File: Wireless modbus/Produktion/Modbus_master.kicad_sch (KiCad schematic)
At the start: 76 parts, among them IC1 LoRa-E5, J1 Screw_Terminal_01x03, J2 XKNANO-113, J3 Conn_01x04_Pin, J4 Conn_Coaxial, J5 Screw_Terminal_01x04, J6 AVR-ISP-6, Q1 BC847CW, Q2 BC847CW, SW1 TL3305AF260QG, U1 ATmega2560-16A, U2 SP485EN-L/TR, U3 L7805, U4 SIM7080G, U5 LSF0204PW-Q100J, Y1 ABM3B-8.000MHZ-10-1-U-T

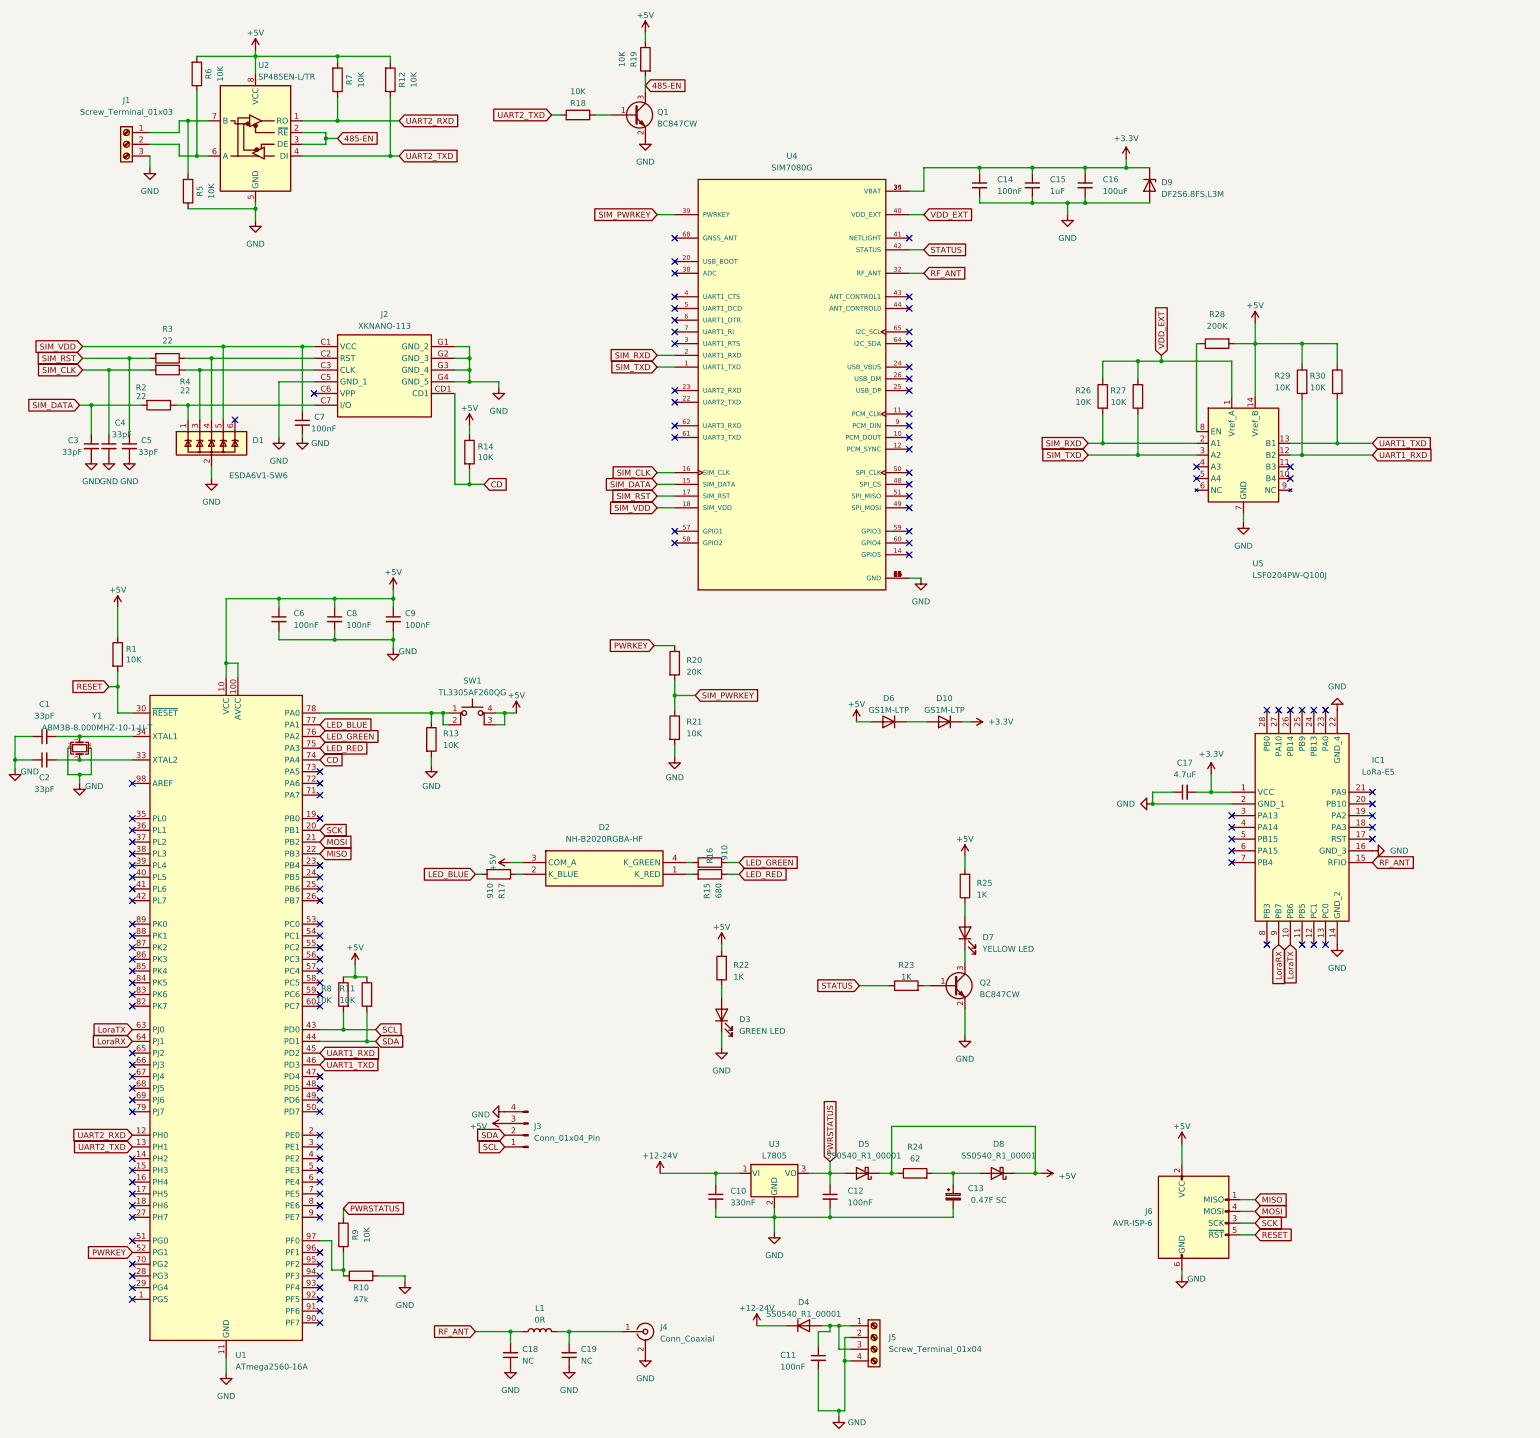
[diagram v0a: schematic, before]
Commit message: Ændring
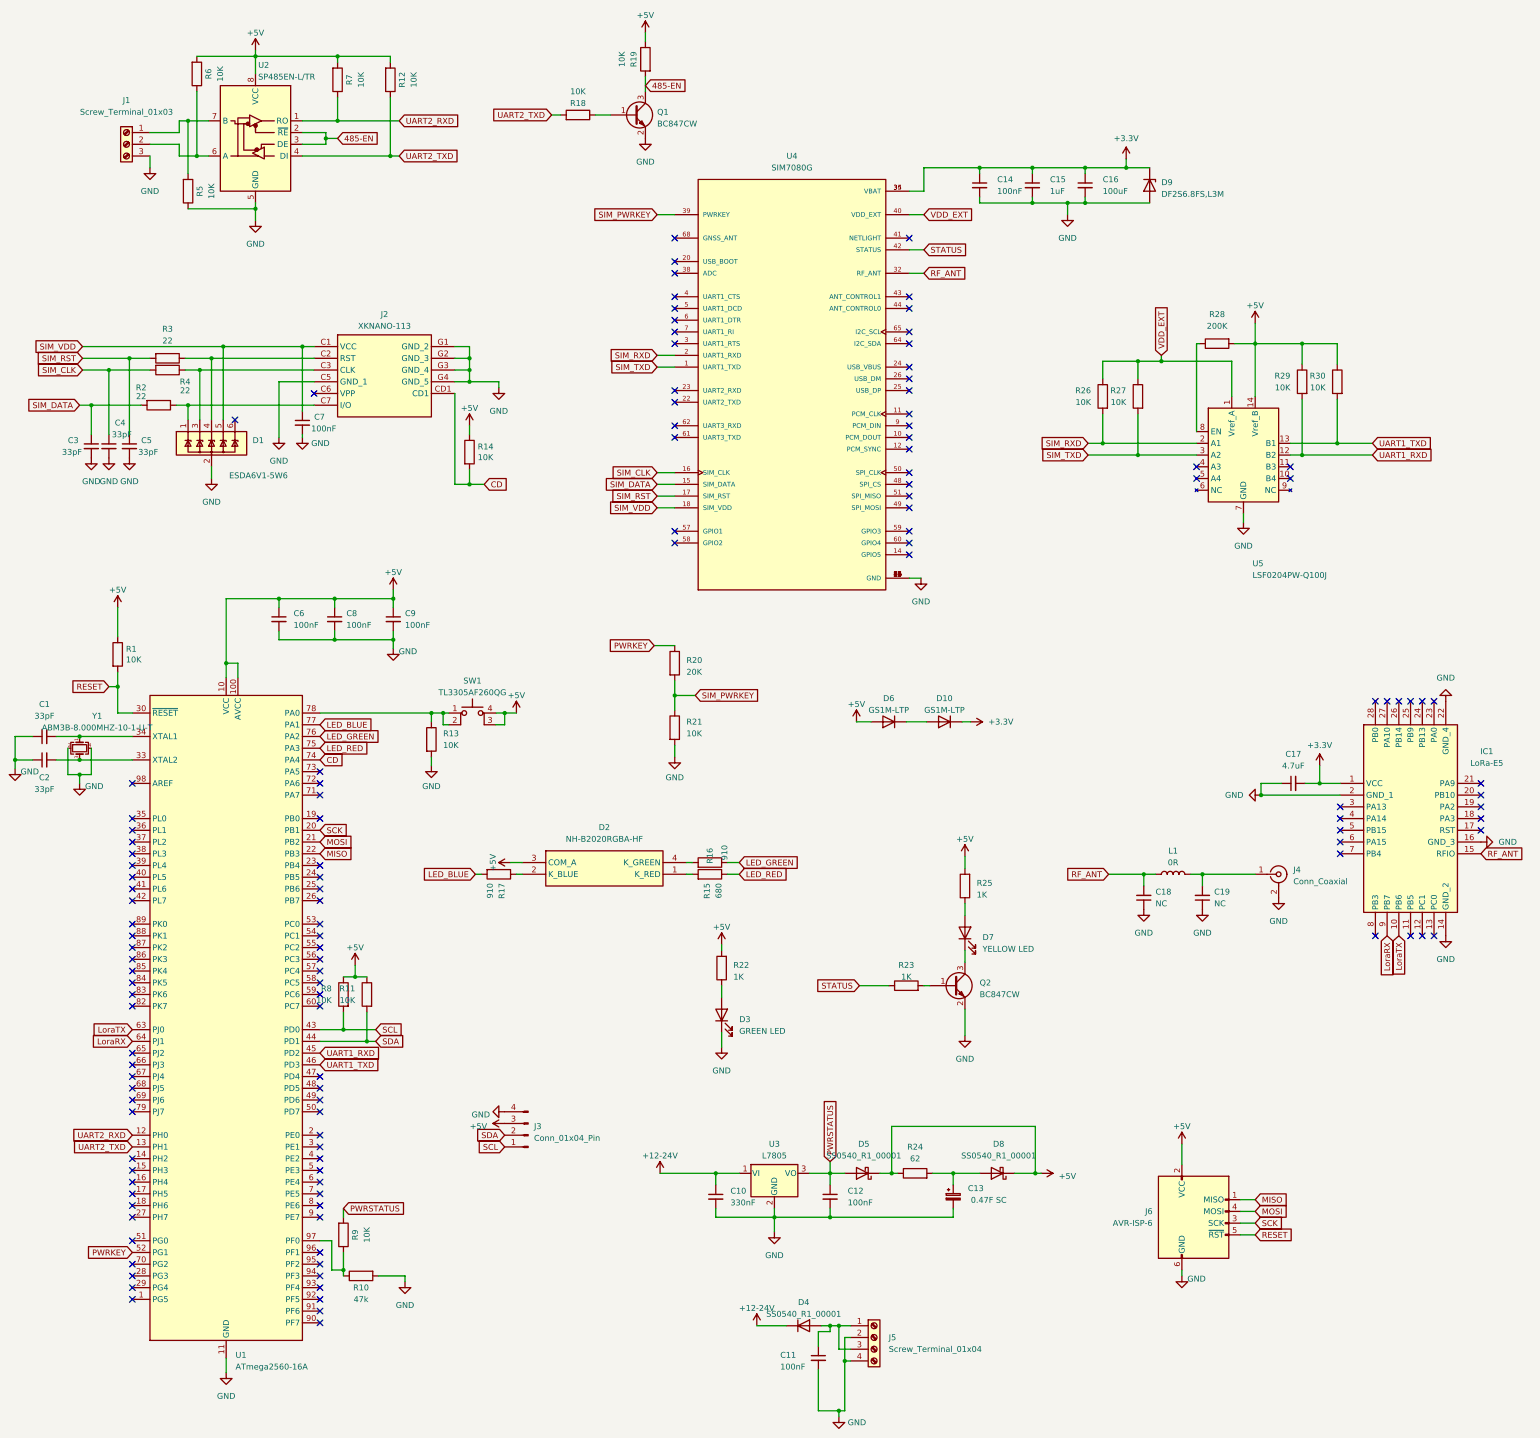
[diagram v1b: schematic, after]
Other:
- moved on the sheet: C17, C18, C19, IC1, J4, L1

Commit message: Ændring
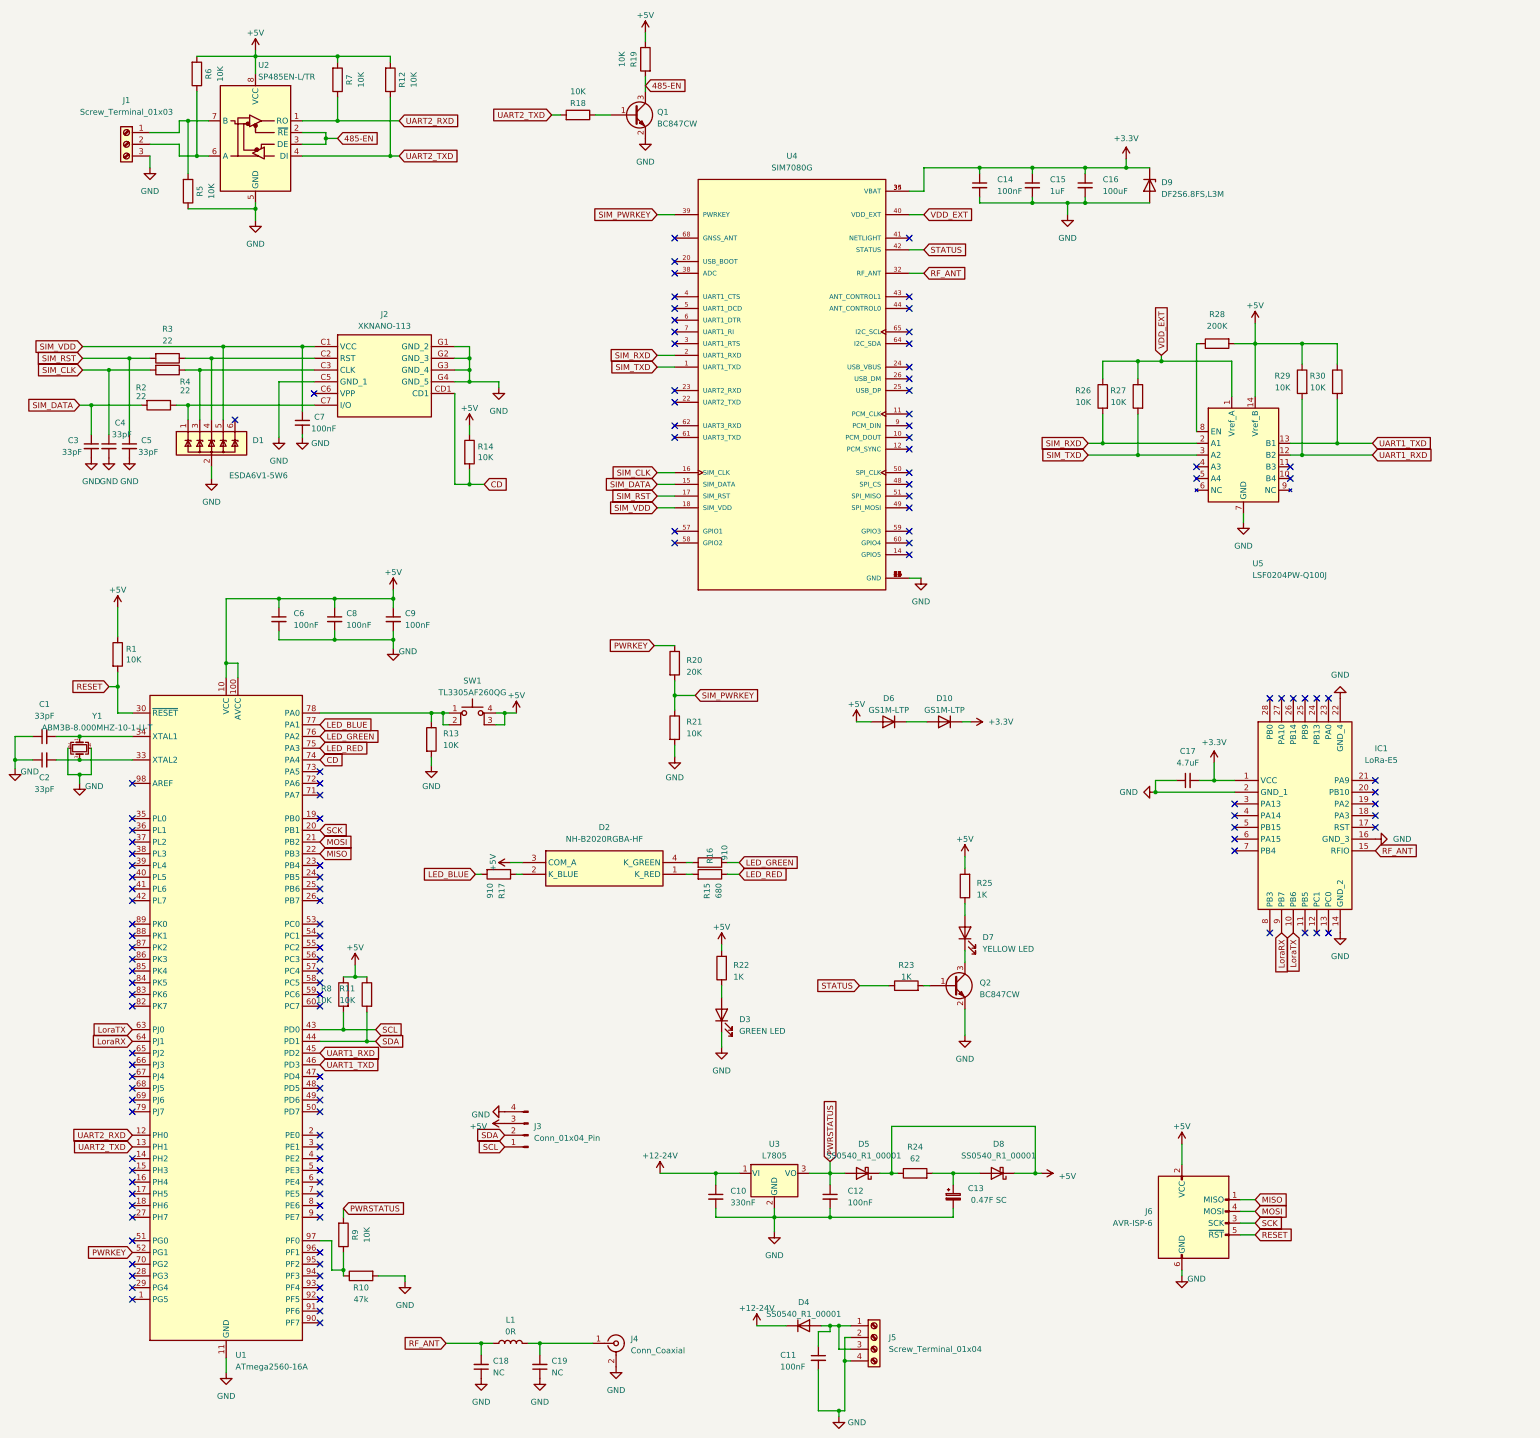
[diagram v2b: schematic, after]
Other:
- moved on the sheet: C17, C18, C19, IC1, J4, L1
